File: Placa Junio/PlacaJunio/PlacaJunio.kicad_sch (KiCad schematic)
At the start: 12 parts, among them J1 Bateria, Q4 IRLML0030, U1 L80-R, U4 MODULO MICRO SD, U5 TSR2-2433N

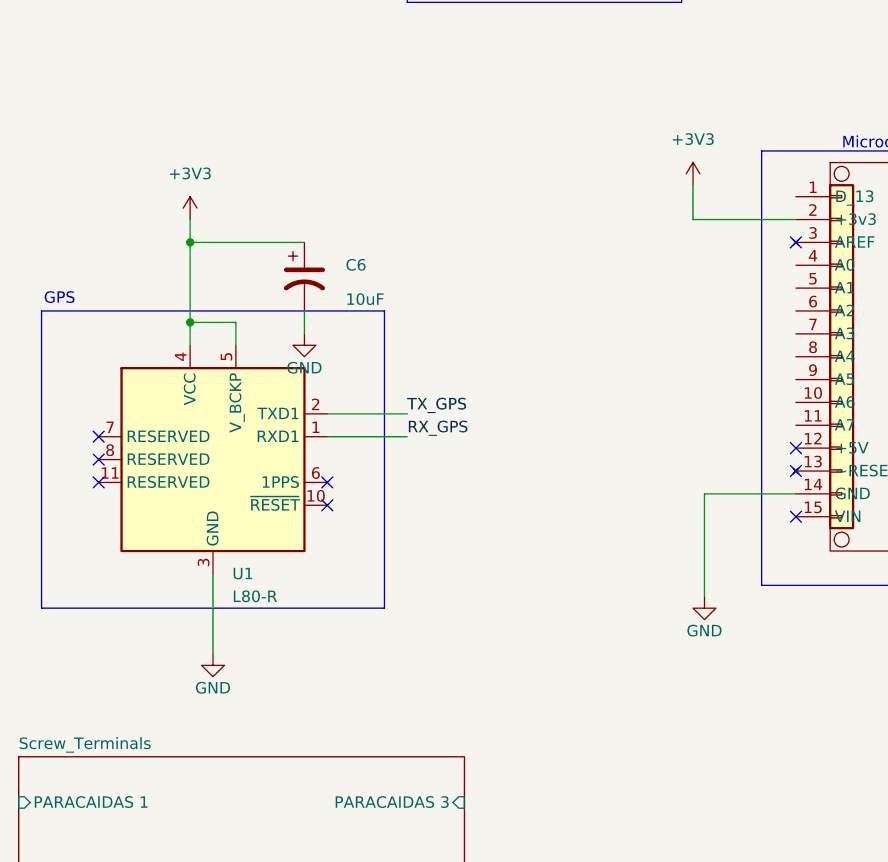
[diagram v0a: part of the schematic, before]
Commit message: Cambios PCB
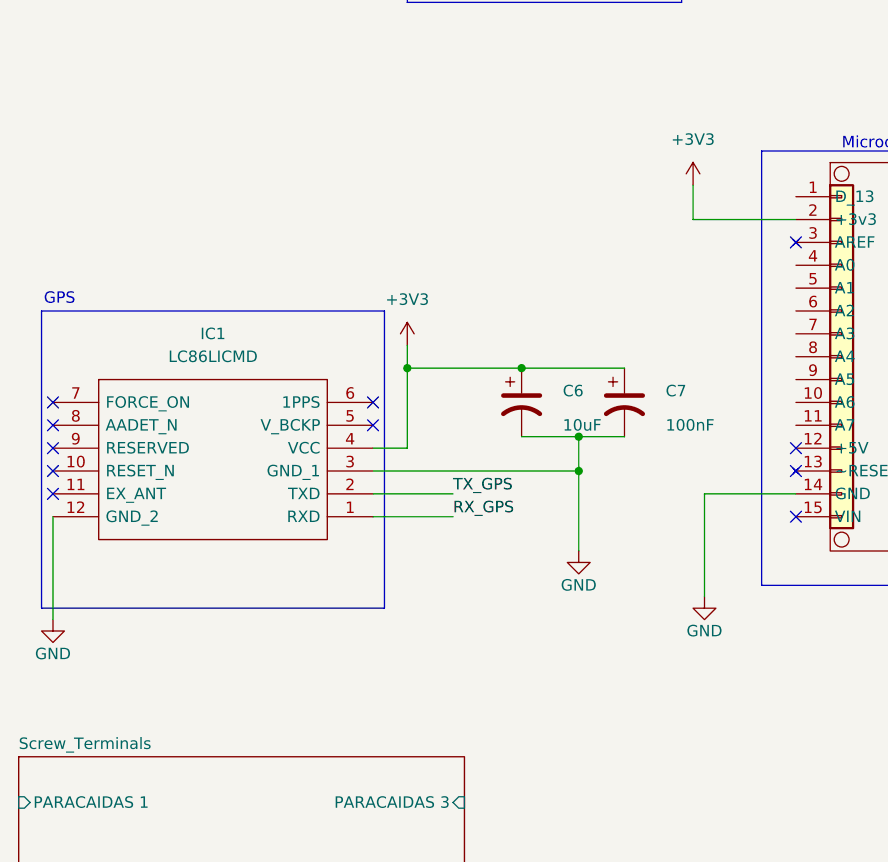
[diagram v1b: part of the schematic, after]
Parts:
- removed U1: L80-R, RF_GPS:Quectel_L80-R, symbol RF_GPS:L80-R
- added C7: 100nF, Capacitor_SMD:C_1206_3216Metric_Pad1.33x1.80mm_HandSolder, symbol Device:C_Polarized_US
- added IC1: LC86LICMD, LC86LICMD, symbol LC86LICMD:LC86LICMD
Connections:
- net +3V3: now also C7.1, IC1.4 (VCC)
- net GND: now also C7.2, IC1.12 (GND_2), IC1.3 (GND_1)
- net RX_GPS: now also IC1.1 (RXD)
- net TX_GPS: now also IC1.2 (TXD)
- no-connect marks 10 -> 12
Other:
- moved on the sheet: C6
